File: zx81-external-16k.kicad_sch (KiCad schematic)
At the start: 10 parts, among them J1 Connector ZX81, U1 CY62256-70PC, U2 74LS00

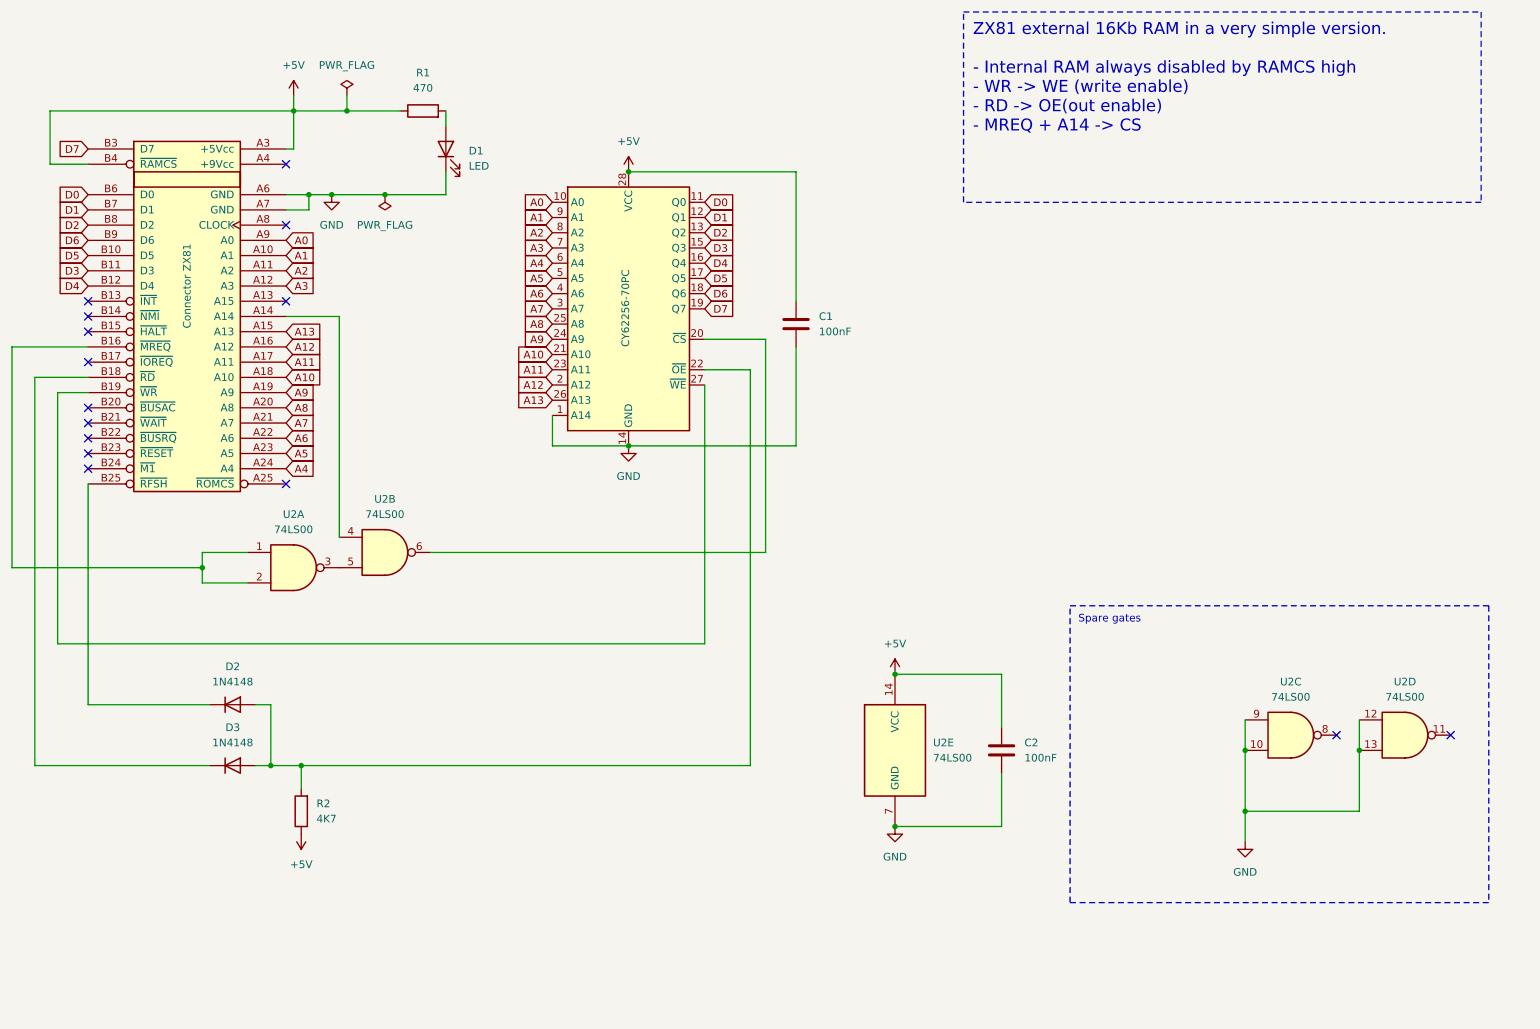
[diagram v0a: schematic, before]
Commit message: v1.1
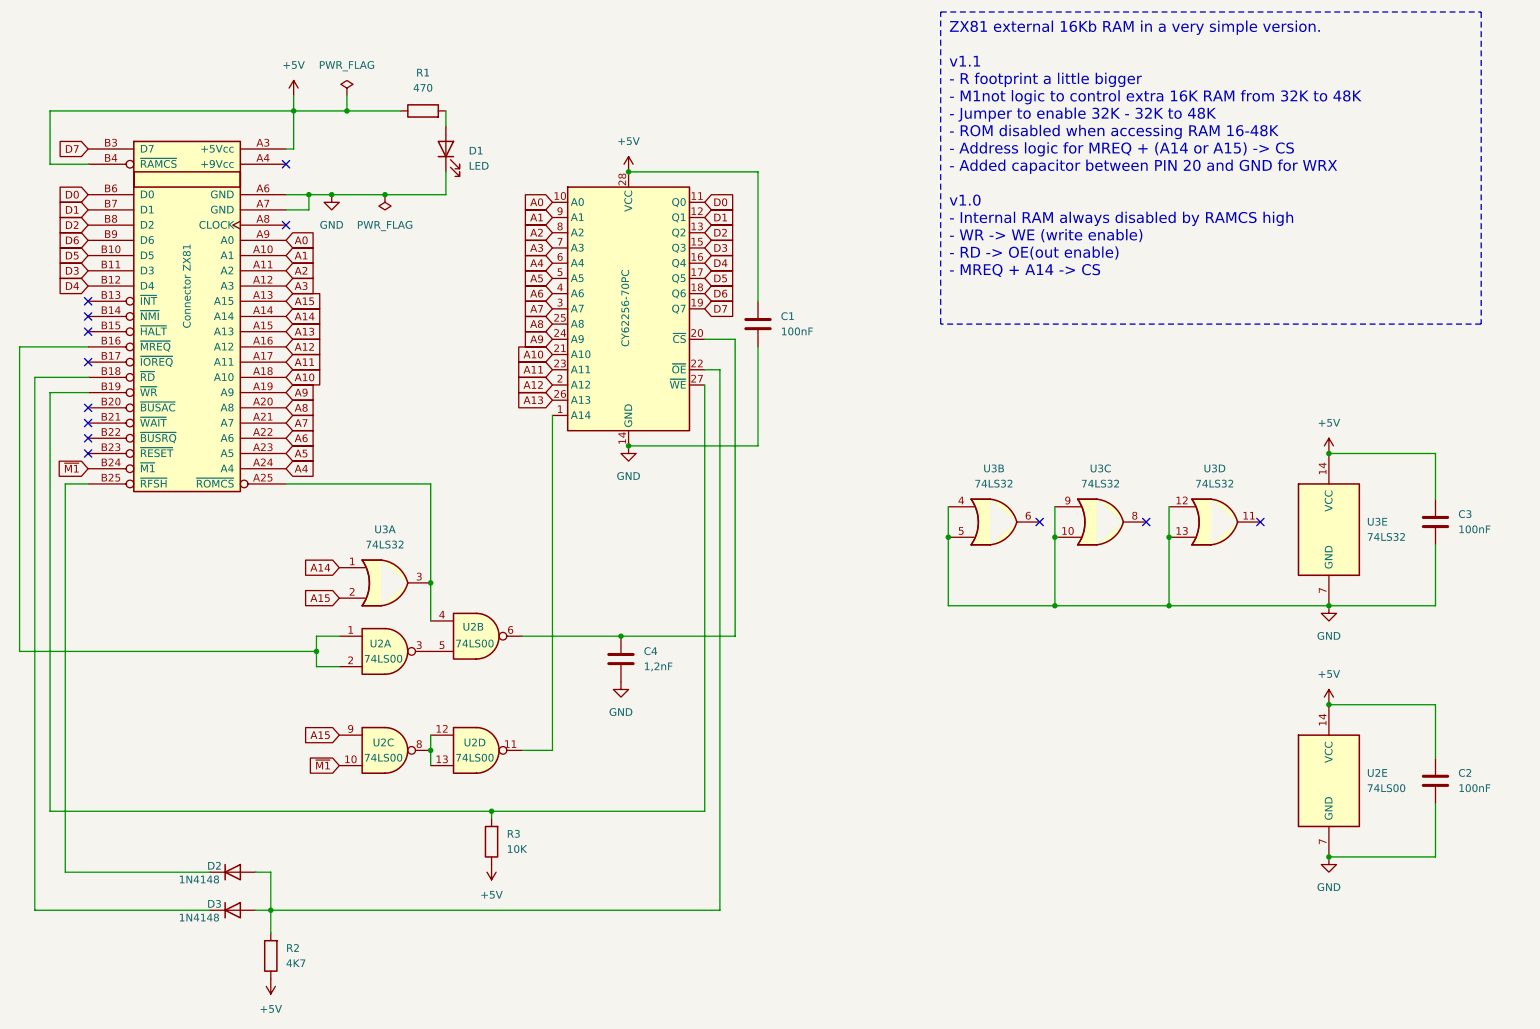
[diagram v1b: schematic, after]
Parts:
- added C3: 100nF, Capacitor_THT:C_Disc_D3.0mm_W1.6mm_P2.50mm, symbol Device:C
- added C4: 1,2nF, Capacitor_THT:C_Disc_D3.0mm_W1.6mm_P2.50mm, symbol Device:C
- added R3: 10K, R_Axial_DIN0207_L6.3mm_D2.5mm_P10.16mm_Horizontal, symbol Device:R
- added U3: 74LS32, Package_DIP:DIP-14_W7.62mm, symbol 74xx:74LS32
- R1, R2: footprint Resistor_THT:R_Axial_DIN0204_L3.6mm_D1.6mm_P5.08mm_Horizontal -> R_Axial_DIN0207_L6.3mm_D2.5mm_P10.16mm_Horizontal
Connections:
- net +5V: now also C3.1, R3.1, U3.14 (VCC)
- net GND: now also C3.2, C4.2, U3.10, U3.12, U3.13, U3.4, U3.5, U3.7 (GND), U3.9; no longer U1.1 (A14), U2.10, U2.12, U2.13, U2.9
- net at U1.20 (~{CS}), U2.6: now also C4.1
- net at J1.B19 (~{WR}), U1.27 (~{WE}): now also R3.2
- net at U2.8: now also U2.12, U2.13
- net A15: now reaches J1.A13 (A15)
- net A15: now also U2.9, U3.2
- net at U2.4: now also J1.A25 (~{ROMCS}), U3.3; no longer J1.A14
- net ~{M1}: now reaches J1.B24 (~{M1})
- net ~{M1}: now also U2.10
- net at U2.11: now also U1.1 (A14)
- new net A14: J1.A14, U3.1
- no-connect marks 15 -> 13
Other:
- note removed: "Spare gates"
- moved on the sheet: C1, C2, D2, D3, R2, U2A, U2B, U2C, U2D, U2E
